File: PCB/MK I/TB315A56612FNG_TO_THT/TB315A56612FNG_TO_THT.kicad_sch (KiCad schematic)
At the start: 44 parts, among them J1 Conn_01x06_Pin, J2 Conn_01x06_Pin, J3 Conn_01x06_Pin, J4 Conn_01x06_Pin, J5 Conn_01x02_Pin, J6 Conn_01x06_Pin, J8 Conn_01x06_Pin, U1 TB6612FNG, U10 QRE1113GR, U11 QRE1113GR, U12 QRE1113GR, U13 QRE1113GR, U2 LM1086, U3 TSOP382xx, U4 DEVKIT_V1_ESP32-WROOM-32, U5 QRE1113GR, U6 QRE1113GR, U7 QRE1113GR, U8 QRE1113GR, U9 QRE1113GR

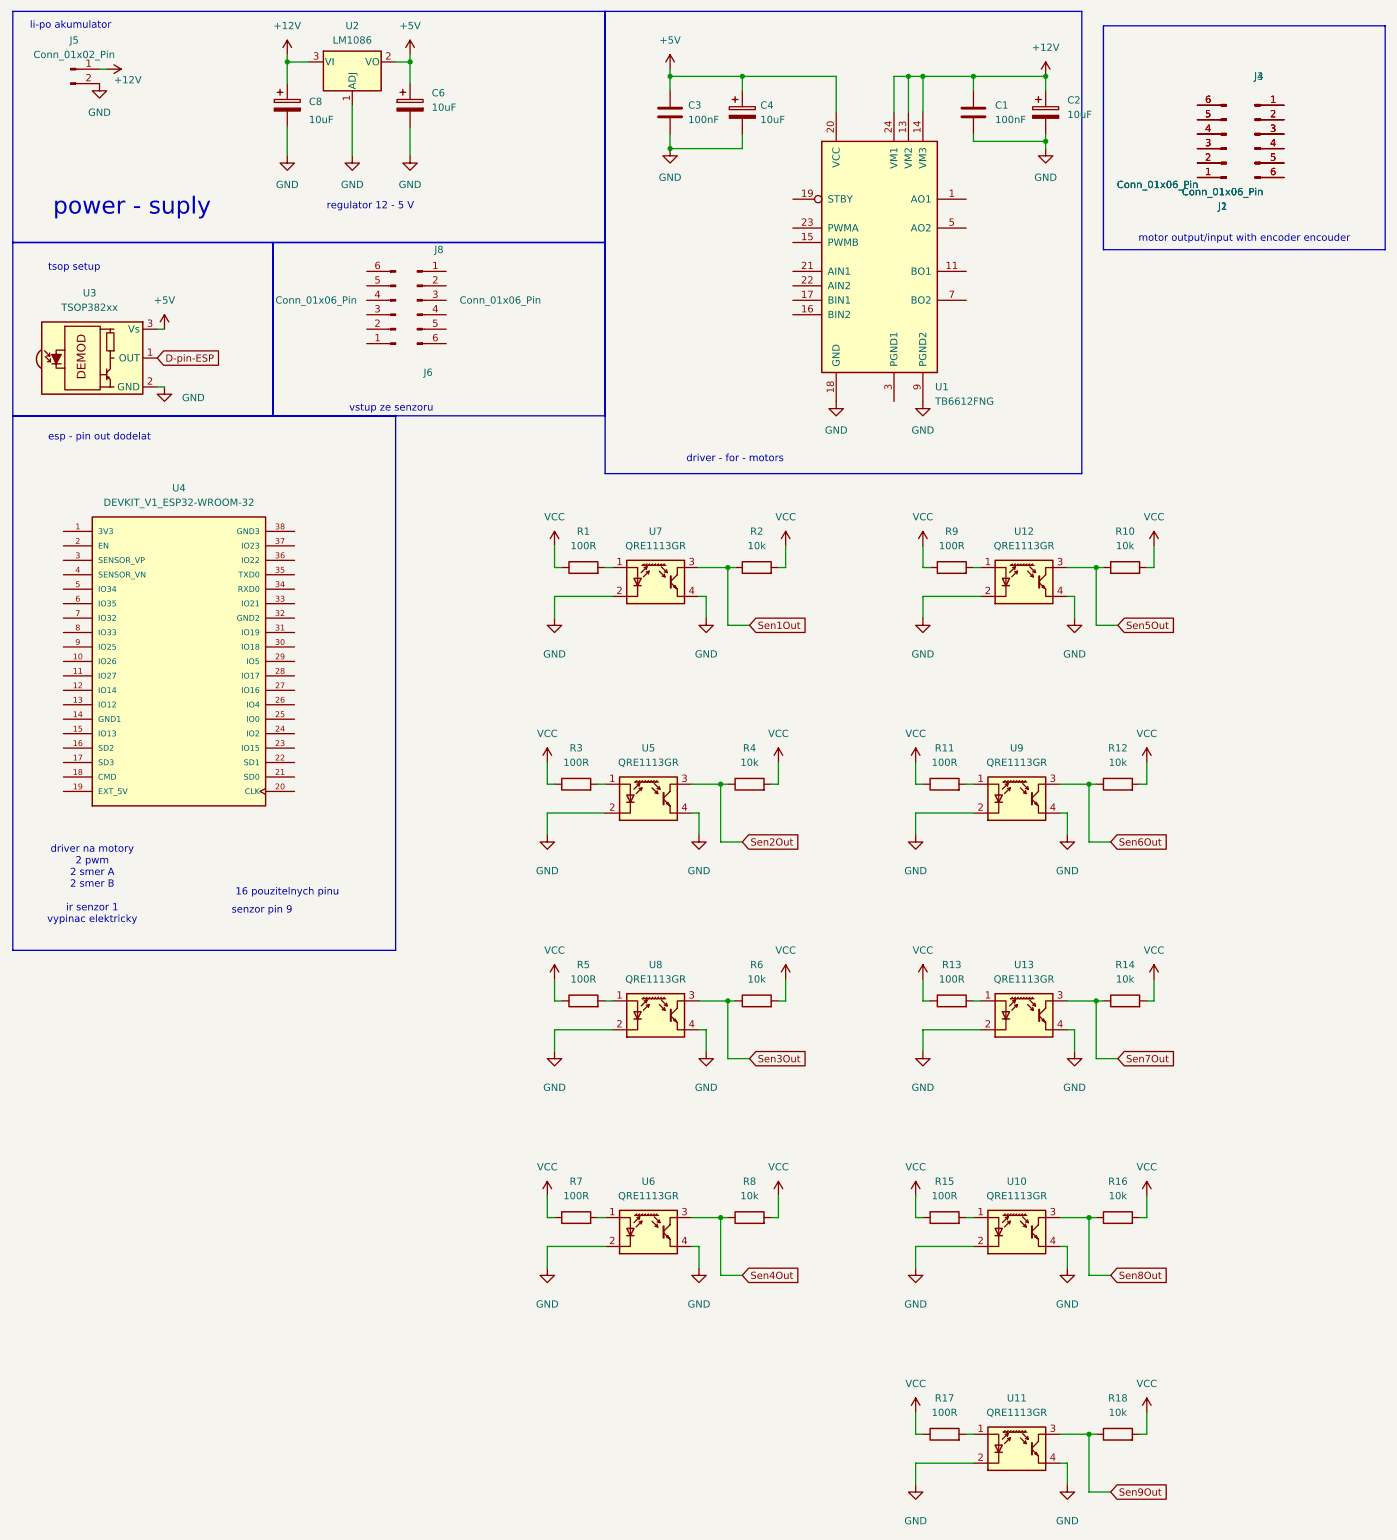
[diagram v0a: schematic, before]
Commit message: ehhh
eeeeh
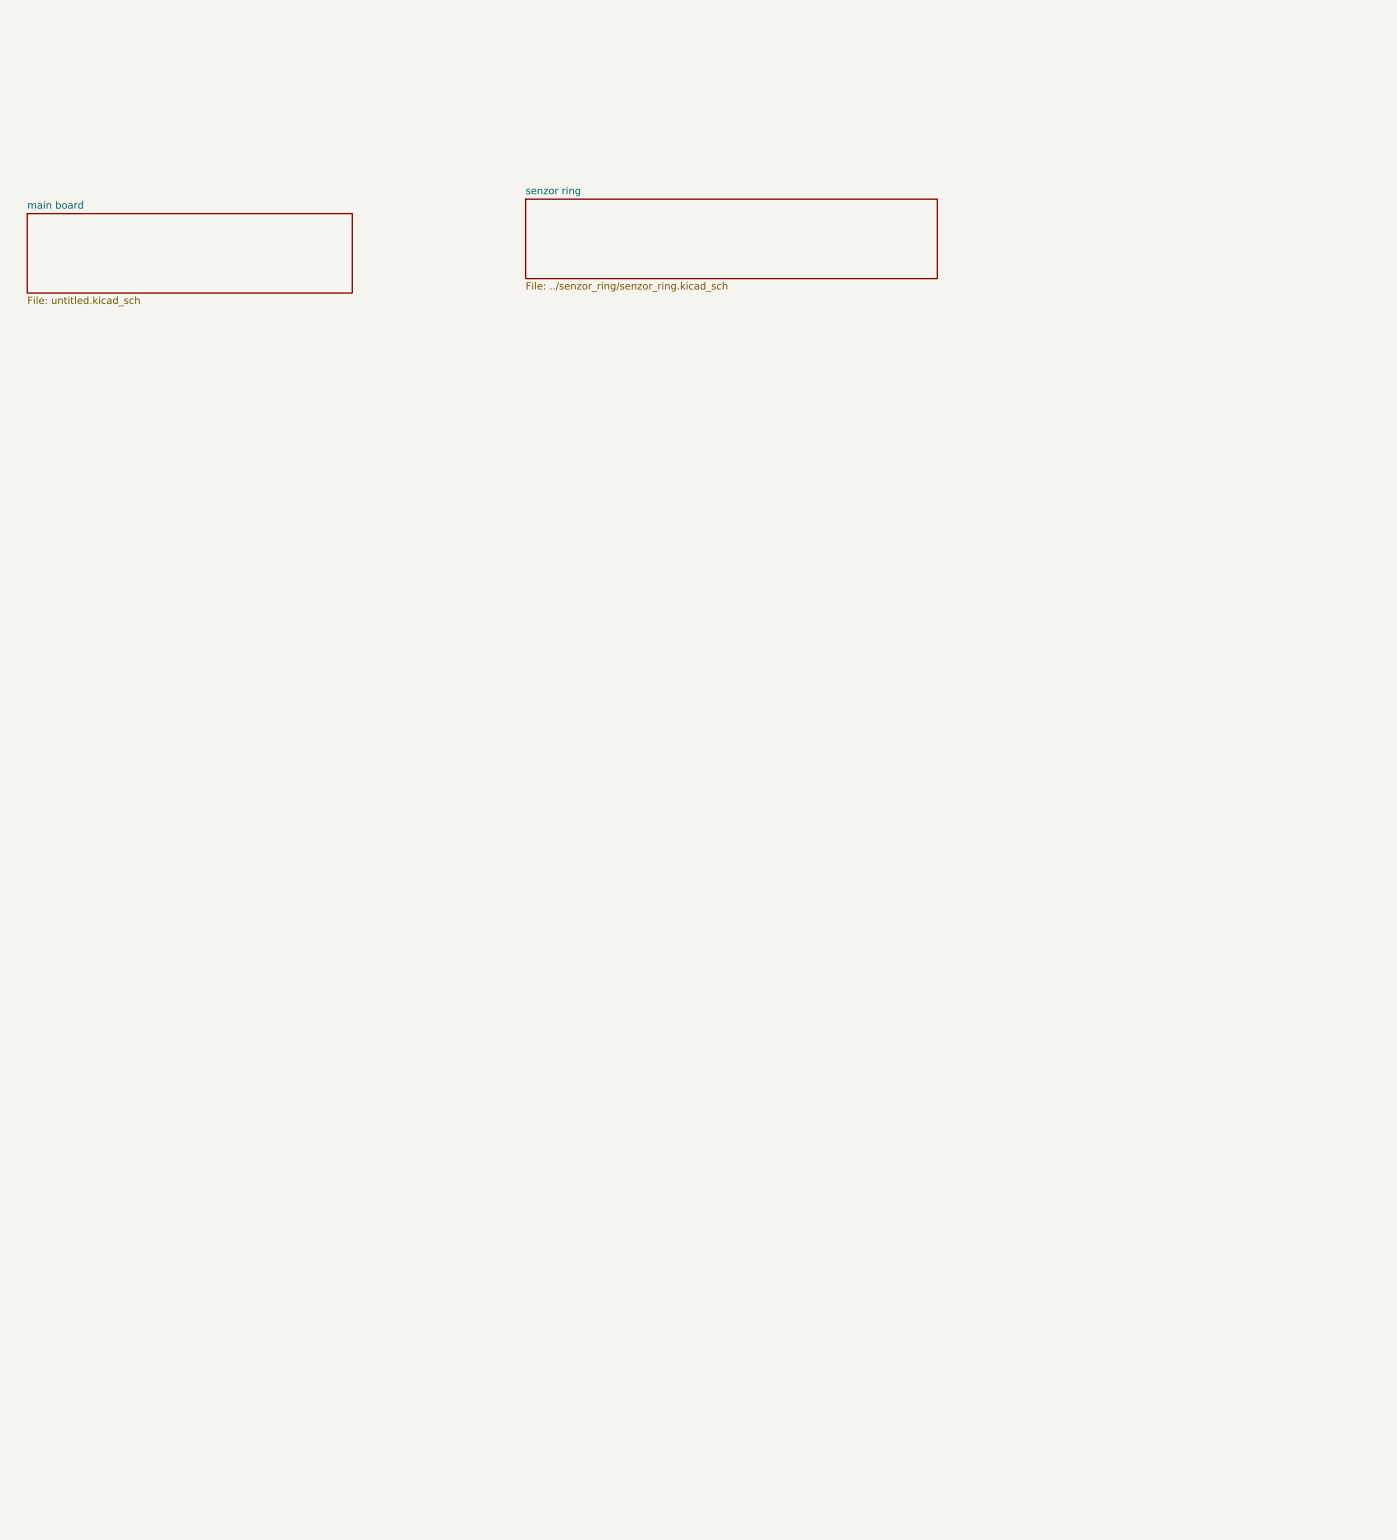
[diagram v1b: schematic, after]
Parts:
- removed C1, C3: 100nF, symbol Device:C
- removed C2, C4, C6, C8: 10uF, symbol Device:C_Polarized
- removed J1, J4: Conn_01x06_Pin, symbol Connector:Conn_01x06_Pin
- removed J2, J3: Conn_01x06_Pin, Connector_JST:JST_SH_BM06B-SRSS-TB_1x06-1MP_P1.00mm_Vertical, symbol Connector:Conn_01x06_Pin
- removed J5: Conn_01x02_Pin, symbol Connector:Conn_01x02_Pin
- removed J6, J8: Conn_01x06_Pin, Connector_JST:JST_XH_B6B-XH-A_1x06_P2.50mm_Vertical, symbol Connector:Conn_01x06_Pin
- removed R1, R11, R13, R15, R17, R3, R5, R7, R9: 100R, Resistor_SMD:R_0805_2012Metric, symbol Device:R
- removed R10, R12, R14, R16, R18, R2, R4, R6, R8: 10k, Resistor_SMD:R_0805_2012Metric, symbol Device:R
- removed U1: TB6612FNG, Package_SO:SSOP-24_5.3x8.2mm_P0.65mm, symbol Driver_Motor:TB6612FNG
- removed U10, U11, U12, U13, U5, U6, U7, U8, U9: QRE1113GR, OptoDevice:OnSemi_CASE100CY, symbol Sensor_Proximity:QRE1113GR
- removed U2: LM1086, Package_TO_SOT_THT:TO-220-3_Vertical, symbol Regulator_Linear:LM317_TO-220
- removed U3: TSOP382xx, OptoDevice:Vishay_MINICAST-3Pin, symbol Interface_Optical:TSOP382xx
- removed U4: DEVKIT_V1_ESP32-WROOM-32, lf_zetor_board:MODULE_DEVKIT_V1_ESP32-WROOM-32, symbol lf_zetor_kicad_sch:DEVKIT_V1_ESP32-WROOM-32
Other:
- added sheet main board (untitled.kicad_sch)
- added sheet senzor ring (../senzor_ring/senzor_ring.kicad_sch)
- note removed: "16 pouzitelnych pinu"
- note removed: "driver - for - motors"
- note removed: "driver na motory 2 pwm 2 smer A 2 smer B"
- note removed: "esp - pin out dodelat"
- note removed: "ir senzor 1 vypinac elektricky"
- note removed: "li-po akumulator"
- note removed: "motor output/input with encoder encouder"
- note removed: "power - suply"
- note removed: "regulator 12 - 5 V"
- note removed: "senzor pin 9"
- note removed: "tsop setup"
- note removed: "vstup ze senzoru"
